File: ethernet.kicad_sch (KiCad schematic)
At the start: 2 parts, among them J1 SI-52008-F, U2 LAN8742A

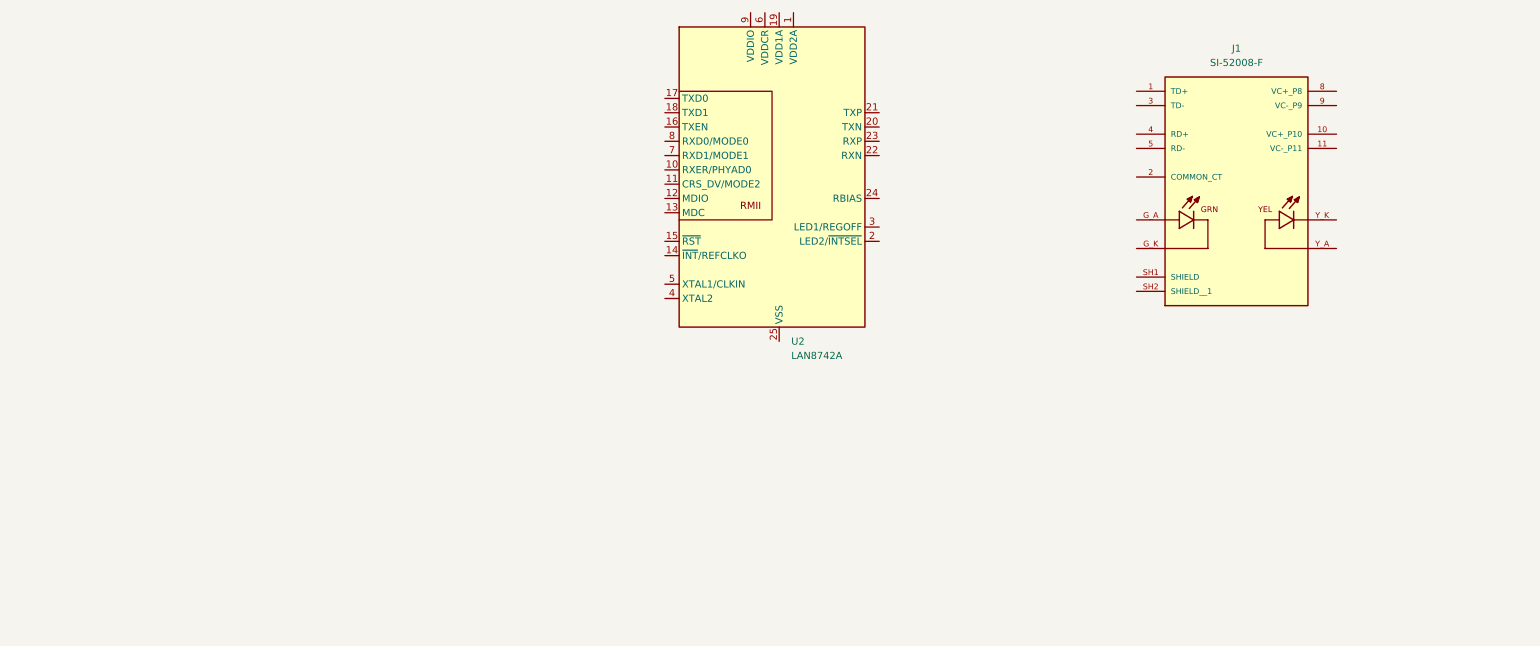
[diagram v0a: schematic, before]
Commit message: Worked on ETH
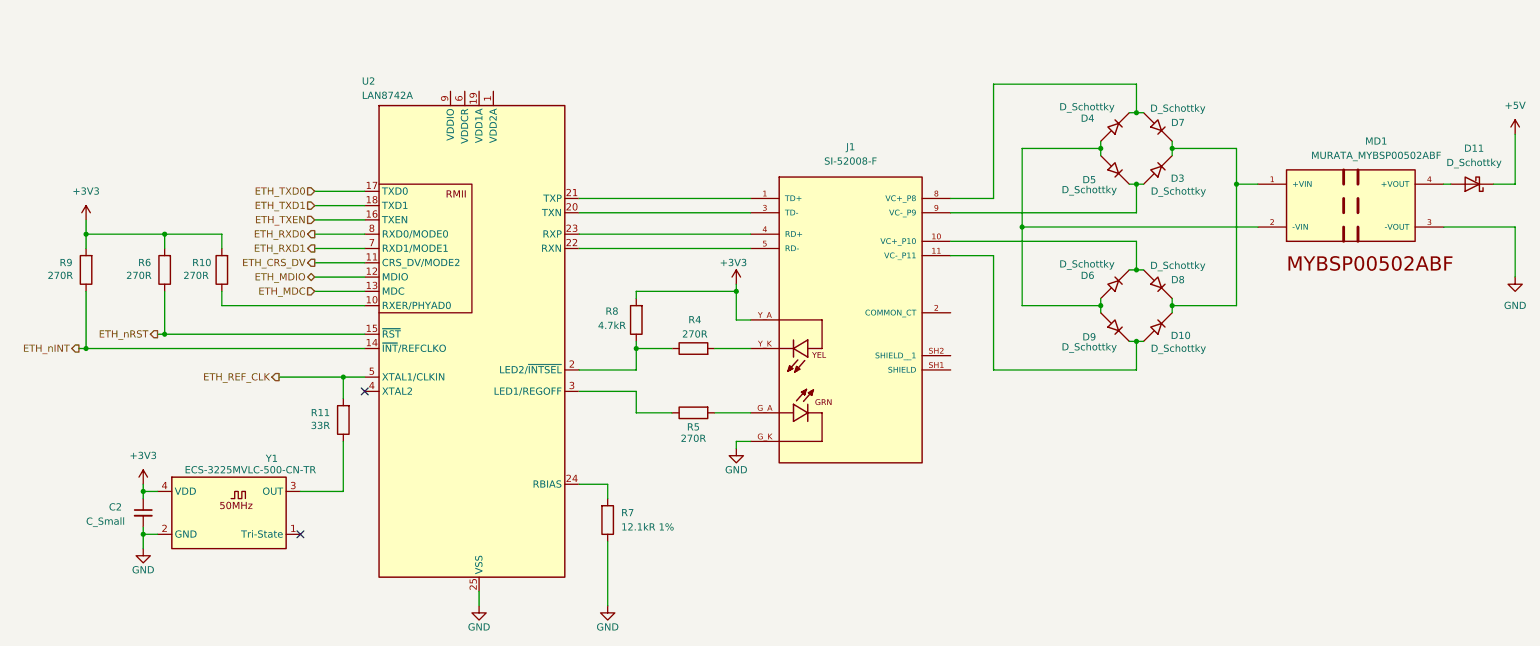
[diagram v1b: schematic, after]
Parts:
- added C2: C_Small, symbol Device:C_Small
- added D10, D3, D4, D5, D6, D7, D8, D9: D_Schottky, symbol Device:D_45deg
- added D11: D_Schottky, Diode_SMD:D_SMA, symbol Device:D_Schottky
- added MD1: MURATA_MYBSP00502ABF, MURATA_MYBSP00502ABF:MURATA_MYBSP00502ABF_0, symbol MURATA_MYBSP00502ABF:MURATA_MYBSP00502ABF
- added R10, R4, R5, R6, R9: 270R, symbol Device:R
- added R11: 33R, symbol Device:R
- added R7: 12.1kR 1%, symbol Device:R
- added R8: 4.7kR, symbol Device:R
- added Y1: ECS-3225MVLC-500-CN-TR, Oscillator:Oscillator_SMD_ECS_2520MV-xxx-xx-4Pin_2.5x2.0mm, symbol Oscillator:ECS-2520MV-xxx-xx
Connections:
- net at U2.10 (RXER/PHYAD0): now also R10.1
- net ETH_CRS_DV: now reaches U2.11 (CRS_DV/MODE2)
- net ETH_MDIO: now reaches U2.12 (MDIO)
- net ETH_MDC: now reaches U2.13 (MDC)
- net ETH_nINT: now reaches U2.14 (~{INT}/REFCLKO)
- net ETH_nINT: now also R9.1
- net ETH_nRST: now reaches U2.15 (~{RST})
- net ETH_nRST: now also R6.1
- net ETH_TXEN: now reaches U2.16 (TXEN)
- net ETH_TXD0: now reaches U2.17 (TXD0)
- net ETH_TXD1: now reaches U2.18 (TXD1)
- net at U2.2 (LED2/~{INTSEL}): now also R4.1, R8.1
- net at U2.20 (TXN): now also J1.3 (TD-)
- net at U2.21 (TXP): now also J1.1 (TD+)
- net at U2.22 (RXN): now also J1.5 (RD-)
- net at U2.23 (RXP): now also J1.4 (RD+)
- net at U2.24 (RBIAS): now also R7.2
- net GND: now reaches U2.25 (VSS)
- net GND: now also J1.G_K, C2.2, MD1.3 (-VOUT), R7.1, Y1.2 (GND)
- net at U2.3 (LED1/REGOFF): now also R5.1
- net ETH_REF_CLK: now reaches U2.5 (XTAL1/CLKIN)
- net ETH_REF_CLK: now also R11.2
- net ETH_RXD1: now reaches U2.7 (RXD1/MODE1)
- net ETH_RXD0: now reaches U2.8 (RXD0/MODE0)
- net at J1.10 (VC+_P10): now also D6.1 (K), D8.2 (A)
- net at J1.11 (VC-_P11): now also D10.2 (A), D9.1 (K)
- net at J1.8 (VC+_P8): now also D4.1 (K), D7.2 (A)
- net at J1.9 (VC-_P9): now also D3.2 (A), D5.1 (K)
- net at J1.G_A: now also R5.2
- net +3V3: now reaches J1.Y_A
- net +3V3: now also C2.1, R10.2, R6.2, R8.2, R9.2, Y1.4 (VDD)
- net at J1.Y_K: now also R4.2
- new net: D4.2 (A), D5.2 (A), D6.2 (A), D9.2 (A), MD1.2 (-VIN)
- new net: R11.1, Y1.3 (OUT)
- new net: D10.1 (K), D3.1 (K), D7.1 (K), D8.1 (K), MD1.1 (+VIN)
- new net: D11.2 (A), MD1.4 (+VOUT)
- new net +5V: D11.1 (K)
- no-connect marks 0 -> 2
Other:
- moved on the sheet: J1, U2
